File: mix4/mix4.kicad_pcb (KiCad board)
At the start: 2 copper layers, 89.8 x 128.5 mm, 33 parts, among them J1 Input A, J2 Input B, J3 Input C, J4 Input D, J5 Mix Out, J6 Power Connector, U1 TL074

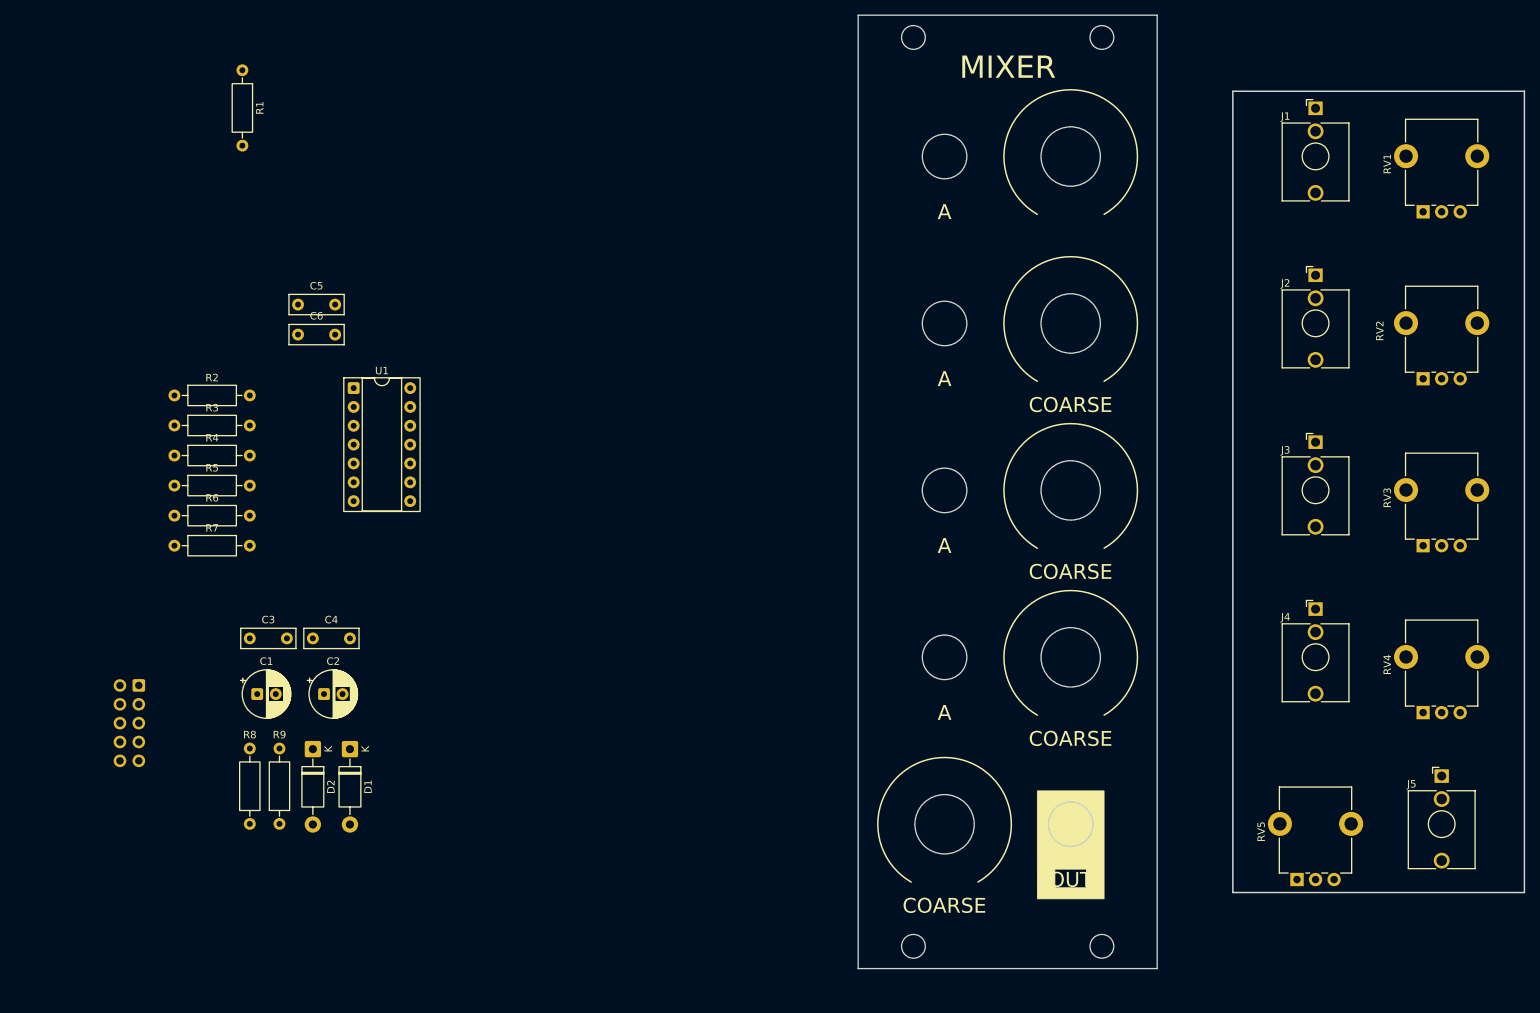
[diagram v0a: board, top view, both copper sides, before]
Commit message: mixer pcb almost done :)
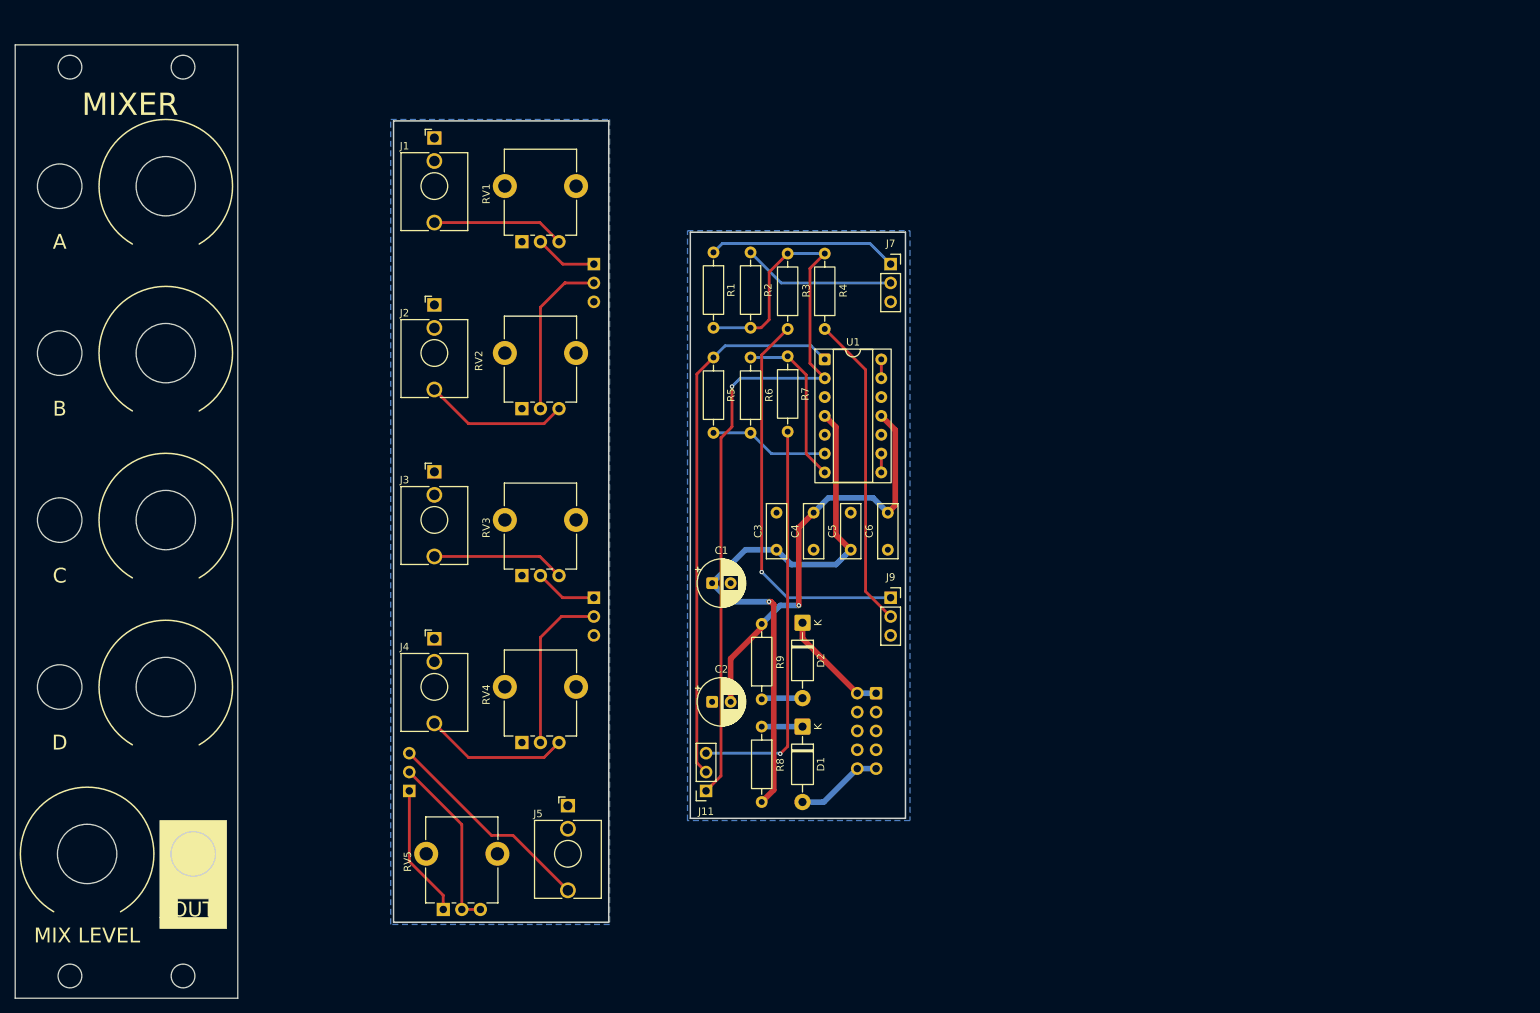
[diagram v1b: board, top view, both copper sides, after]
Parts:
- added J10: ~, Connector_PinHeader_2.54mm:PinHeader_1x03_P2.54mm_Vertical, B.Cu at (108.0, 136.0)
- added J11: Conn_01x03, Connector_PinSocket_2.54mm:PinSocket_1x03_P2.54mm_Vertical, F.Cu at (148.0, 136.0)
- added J6: Conn_01x03, Connector_PinHeader_2.54mm:PinHeader_1x03_P2.54mm_Vertical, B.Cu at (132.9, 65.0)
- added J7: ~, Connector_PinSocket_2.54mm:PinSocket_1x03_P2.54mm_Vertical, F.Cu at (172.9, 65.0)
- added J8: Conn_01x03, Connector_PinHeader_2.54mm:PinHeader_1x03_P2.54mm_Vertical, B.Cu at (132.9, 110.0)
- added J9: ~, Connector_PinSocket_2.54mm:PinSocket_1x03_P2.54mm_Vertical, F.Cu at (172.9, 110.0)
- moved REF** 123.9 mm to (77.5, 161.0)
- moved REF** 123.9 mm to (77.5, 38.5)
- moved RV1 121.5 mm to (123.2, 62.0)
- moved RV2 121.5 mm to (123.2, 84.5)
- moved RV3 121.5 mm to (123.2, 107.0)
- moved RV4 121.5 mm to (123.2, 129.5)
- moved J1 118.8 mm to (111.4, 48.0)
- moved J2 118.8 mm to (111.4, 70.5)
- moved J3 118.8 mm to (111.4, 93.0)
- moved J4 118.8 mm to (111.4, 115.5)
- moved J5 117.8 mm to (129.4, 138.0)
- moved RV5 115.1 mm to (112.6, 152.0)
- moved REF** 113.8 mm to (62.3, 161.0)
- moved REF** 113.8 mm to (62.3, 38.5)
- moved J12 99.4 mm to (170.9, 122.8)
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- renumbered J6 to J12
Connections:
- net Net-(J5-PadT) renamed MIX_OUT
- net Net-(R1-Pad1) renamed INPUT_A
- net Net-(R2-Pad1) renamed INPUT_B
- net Net-(R3-Pad1) renamed INPUT_C
- net Net-(R4-Pad1) renamed INPUT_D
- net Net-(R5-Pad1) renamed MIX_GAIN_2
- net Net-(U1A--) renamed MIX_GAIN_1
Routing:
- net MIX_GAIN_1: track 0.00 -> 128.2 mm, vias 0 -> 1
- net MIX_GAIN_2: track 0.00 -> 97.7 mm
- net MIX_OUT: track 0.00 -> 82.9 mm, vias 0 -> 1
- net +12V: track 0.00 -> 78.7 mm, vias 0 -> 1
- net INPUT_D: track 0.00 -> 65.0 mm
- net INPUT_C: track 0.00 -> 61.5 mm, vias 0 -> 1
- net -12V: track 0.00 -> 57.5 mm, vias 0 -> 1
- net INPUT_B: track 0.00 -> 42.8 mm
- net INPUT_A: track 0.00 -> 34.0 mm
- net Net-(R6-Pad2): track 0.00 -> 22.8 mm
- net Net-(J4-PadT): track 0.00 -> 19.5 mm
- net Net-(J2-PadT): track 0.00 -> 19.5 mm
- net Net-(J1-PadT): track 0.00 -> 17.9 mm
- net Net-(J3-PadT): track 0.00 -> 17.9 mm
- net Net-(U1B--): track 0.00 -> 16.2 mm
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- added copper zone on B.Cu, net GND
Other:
- board size 89.8 x 128.5 mm -> 120 x 128.5 mm
- board text added: "B"
- board text added: "C"
- board text added: "D"
- board text added: "MIX LEVEL"
- board text removed: "COARSE"
